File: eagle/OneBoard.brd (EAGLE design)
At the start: 52 x 70.8 mm, 29 parts

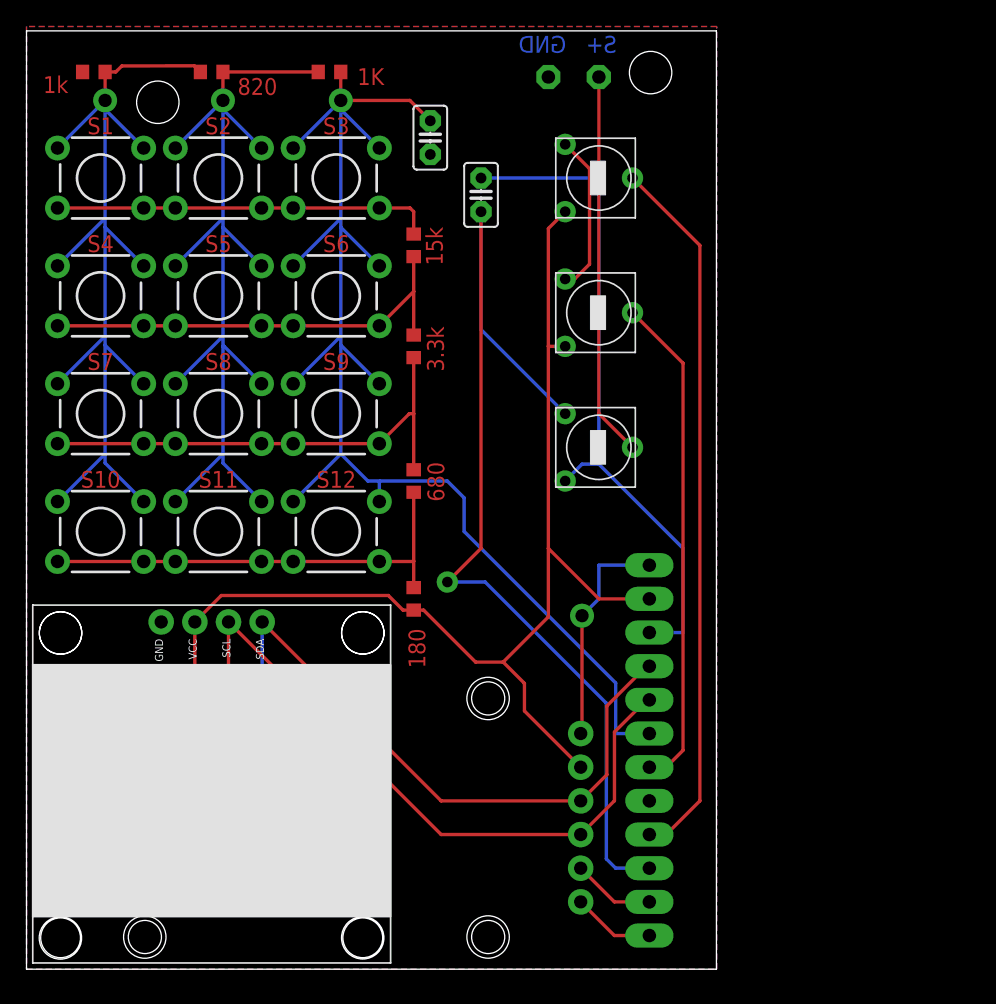
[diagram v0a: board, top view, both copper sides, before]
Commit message: updated
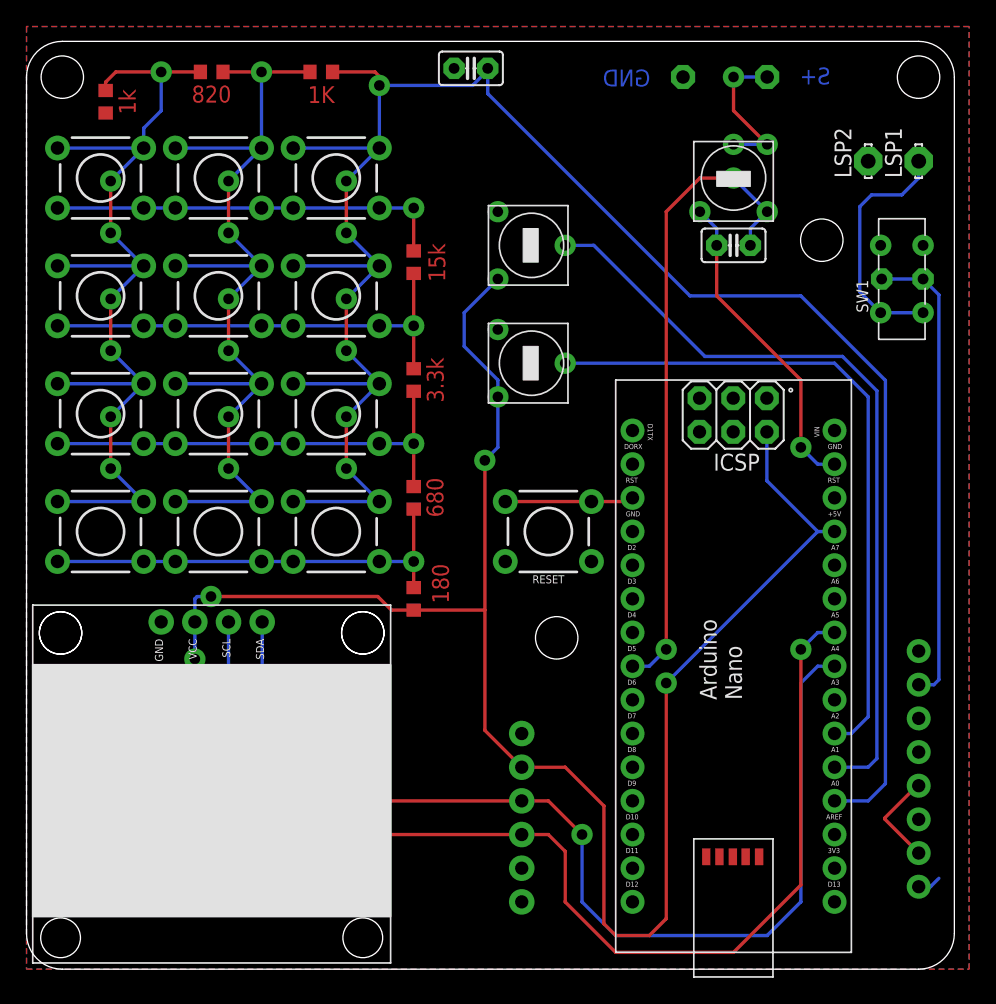
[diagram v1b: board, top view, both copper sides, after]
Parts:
- removed JP1: PINHD-1X12-FEMALE, Pat Sonstiges:1X12-FEMALE
- removed U$2: (no value), My Breakout Boards:DS3231_BREAKOUT
- added LSP1, LSP2: LSP11, solpad:LSP11
- added POWERBOOST: ADAFRUIT_POWERBOOST_1000C, My Breakout Boards:ADAFRUIT_POWERBOOST_1000C
- added RESET: TACTILE_BUTTON_6X6X9.5, Pat Sonstiges:TACTILE_SWITCH_PTH_6.0MM
- added RTC: (no value), My Breakout Boards:DS3231_BREAKOUT
- added SW1: (no value), Seeed-Switch:SW6-2.54-9.0X3.5X3.2+2.0MM
- added U$7: ARDUINO-NANO, My Boards:ARDUINO_NANO
- moved U$5 22.7 mm to (53.3, 59.7), turned to 0 degrees
- moved C1 19.4 mm to (53.3, 54.6), turned to 180 degrees
- moved S+ 12.7 mm to (55.9, 67.3)
- moved GND 10.2 mm to (49.5, 67.3)
- moved U$4 7.18 mm to (38.1, 54.6)
- moved U$3 6.35 mm to (38.1, 45.7)
- moved C2 6.06 mm to (33.5, 68.0), turned to 0 degrees
- moved R2 2.54 mm to (29.2, 44.5)
- moved R7 2.42 mm to (5.97, 65.4), turned to 90 degrees
- moved R1 1.27 mm to (29.2, 53.3)
- moved R3 1.27 mm to (29.2, 35.6)
- moved R5 0.62 mm to (22.2, 67.7)
- renumbered U$1 to DISPLAY
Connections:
- new net 3V3: U$7.3V3
- new net A6: U$7.A6
- new net A7: U$7.A7
- new net BAT+: LSP1.MP, SW1.CH1A, SW1.CH2A
- new net D10: U$7.D10
- new net D11: U$7.D11
- new net D12: U$7.D12
- new net D13: U$7.D13
- new net D2: U$7.D2
- new net D3: U$7.D3
- new net D4: U$7.D4
- new net D6: U$7.D6
- new net D7: U$7.D7
- new net D8: U$7.D8
- new net D9: U$7.D9
- new net MISO: U$7.MISO
- new net MOSI: U$7.MOSI
- new net N$1: RTC.SDA2
- new net N$2: RTC.SCL2
- new net REF: U$7.REF
- new net RESET..: U$7.RESET..
- new net RST: RESET.3, RESET.4, U$7.RST
- new net RST.: U$7.RST.
- new net RX0: U$7.RX1
- new net SCK: U$7.SCK
- new net TX1: U$7.TX1
- new net VBAT: POWERBOOST.P$2, SW1.COM1, SW1.COM2
- new net VIN_NANO: U$7.VIN
- new net VOUT: POWERBOOST.P$8
- new net VS: POWERBOOST.P$3
- new net VUSB: POWERBOOST.P$1
- net 32K: now also RTC.32K; no longer JP1.1, U$2.32K
- net 5V: now also RTC.VCC1, RTC.VCC2, U$7.5V, U$7.5V.; no longer JP1.11, U$2.VCC1, U$2.VCC2
- net A0: now also C2.2, R5.2, S12.1, S12.2, S3.1, S3.2, S6.1, S6.2, S9.1, S9.2, U$7.A0; no longer JP1.4, U$4.S
- net A1: now also U$4.S, U$7.A1; no longer JP1.5
- net A2: now also U$7.A2; no longer JP1.6
- net A3: now also U$7.A3; no longer C2.2, JP1.7, R5.2, S12.1, S12.2, S3.1, S3.2, S6.1, S6.2, S9.1, S9.2
- net D5: now also U$7.D5; no longer JP1.10
- net GND: now also LSP2.MP, POWERBOOST.P$5, POWERBOOST.P$7, RESET.1, RESET.2, RTC.GND1, RTC.GND2, U$7.GND, U$7.GND_; no longer JP1.12, U$2.GND1, U$2.GND2
- net GND_PWM: now also U$7.GND.; no longer JP1.3
- net SCL: now also RTC.SCL1, U$7.A5; no longer JP1.8, U$2.SCL1, U$2.SCL2
- net SDA: now also RTC.SDA1, U$7.A4; no longer JP1.9, U$2.SDA1, U$2.SDA2
- net SQW: now also RTC.SQW; no longer JP1.2, U$2.SQW
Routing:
- net A3: track 106.9 -> 0.00 mm, vias 1 -> 0
- net A0: track 54.0 -> 152.4 mm, vias 0 -> 7
- net A1: track 0.00 -> 59.3 mm
- net GND_PWM: track 77.9 -> 24.0 mm
- net 5V: track 99.0 -> 148.8 mm, vias 0 -> 4
- net VBAT: track 0.00 -> 35.5 mm
- net GND: track 29.2 -> 7.26 mm, vias 1 -> 0
- net BAT+: track 0.00 -> 18.5 mm
- net S+: track 29.0 -> 11.2 mm, vias 0 -> 2
- net SDA: track 62.8 -> 77.0 mm, vias 0 -> 2
- net SCL: track 67.9 -> 81.8 mm, vias 0 -> 2
- net A2: track 37.7 -> 51.1 mm
- net RST: track 0.00 -> 9.72 mm
- net SQW: track 6.23 -> 0.00 mm
- net 32K: track 6.23 -> 0.00 mm
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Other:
- board size 52 x 70.8 mm -> 70 x 70 mm
